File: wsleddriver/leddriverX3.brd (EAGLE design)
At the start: 100 x 38.1 mm, 55 parts, among them IC1 WS2811-SOP8, IC2 WS2811-SOP8, IC3 WS2811-SOP8

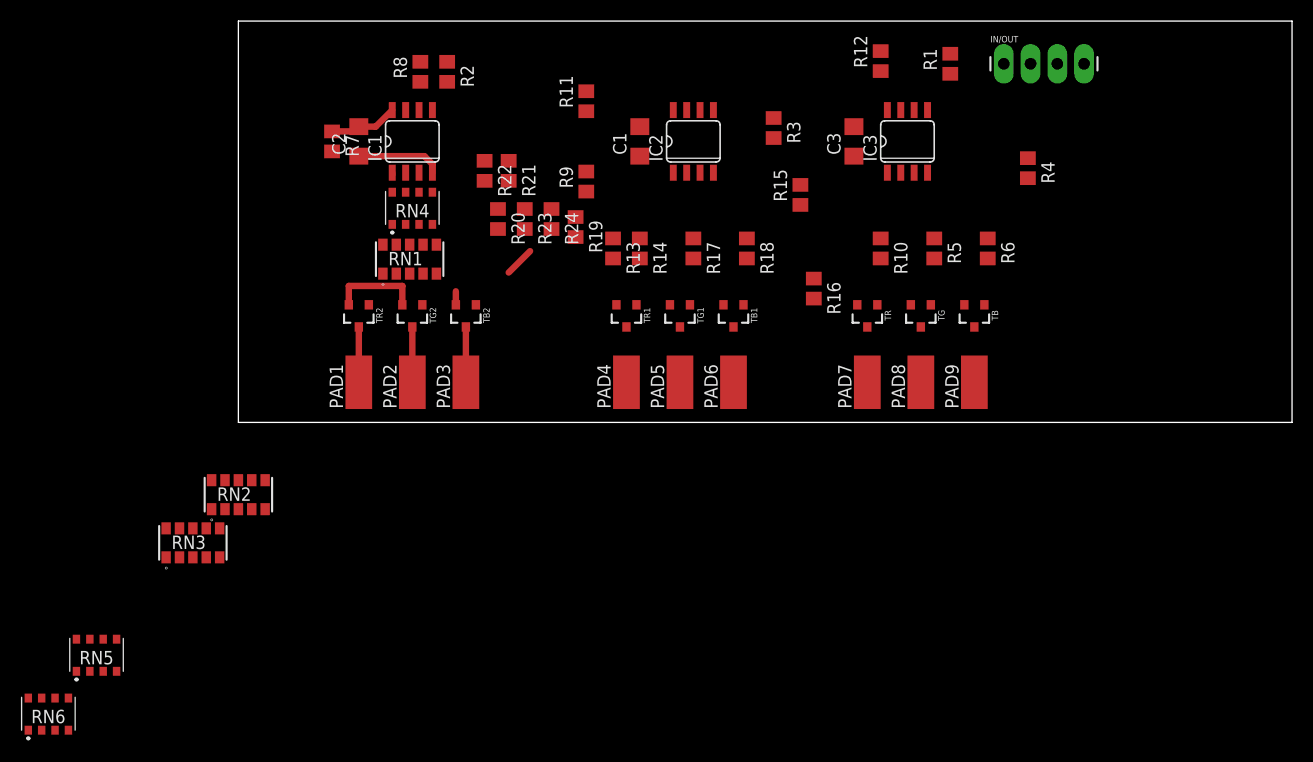
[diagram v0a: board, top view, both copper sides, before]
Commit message: h
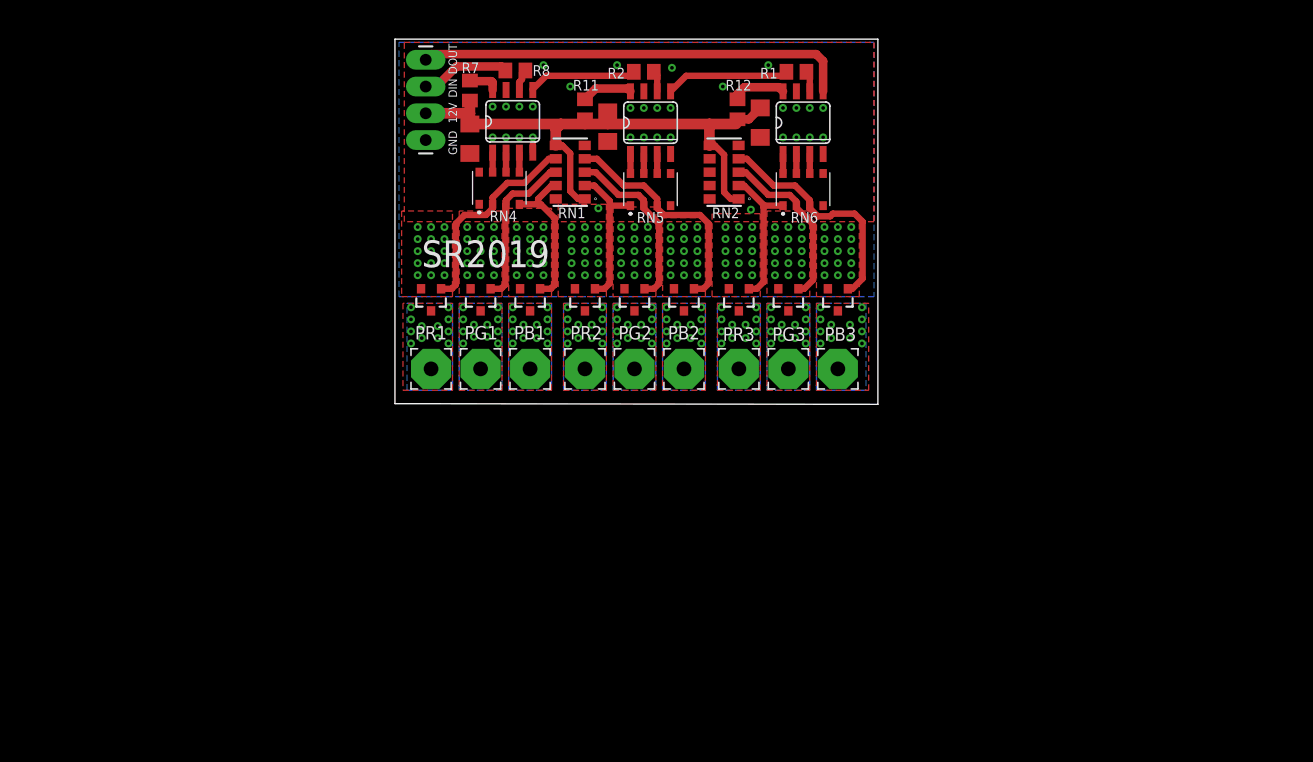
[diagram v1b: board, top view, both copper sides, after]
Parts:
- removed PAD1, PAD2, PAD3, PAD4, PAD5, PAD6, PAD7, PAD8, PAD9: (no value), wirepad:SMD2,54-5,08
- removed R10, R14, R17, R18, R20, R23, R24, R5, R6: 100, rcl:R0805
- removed R13, R15, R16, R19, R21, R22, R3, R4, R9: 10k, rcl:R0805
- removed RN3: YC358TJK-0710KL, SamacSys_Parts:YC358T
- added PB1, PB2, PB3, PG1, PG2, PG3, PR1, PR2, PR3: (no value), wirepad:3,81/1,4
- moved RN6 87.2 mm to (53.6, 22.1)
- moved RN5 68.7 mm to (39.1, 22.1)
- moved IN/OUT 55.3 mm to (17.8, 26.8), turned to 90 degrees
- moved RN2 55.3 mm to (46.1, 23.7), turned to 90 degrees
- moved R2 18.7 mm to (38.5, 33.3), turned to 180 degrees
- moved RN1 17.3 mm to (31.5, 23.7), turned to 90 degrees
- moved R1 14.6 mm to (53.0, 33.3), turned to 180 degrees
- moved R12 14.3 mm to (47.4, 29.7), turned to 270 degrees
- moved R7 13.9 mm to (22.0, 31.5)
- moved TB 13.0 mm to (56.9, 11.7)
- moved TG 12.7 mm to (52.2, 11.7)
- moved TR 12.3 mm to (47.5, 11.7)
- moved C2 10.5 mm to (22.0, 26.9)
- moved IC3 10.1 mm to (53.6, 28.4)
- moved IC1 9.71 mm to (26.0, 28.6)
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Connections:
- removed net N$10: R21.2, R23.2, TG2.1
- removed net N$12: R22.2, R24.2, TB2.1
- removed net N$15: RN1.2, RN1.7, RN4.3
- removed net N$16: RN1.3, RN1.8, RN4.2
- removed net N$17: RN1.4, RN1.9, RN4.1
- removed net N$2: R3.2, R5.2, TG.1
- removed net N$3: R4.2, R6.2, TB.1
- removed net N$4: R10.2, R9.2, TR.1
- removed net N$6: R13.2, R14.2, TR1.1
- removed net N$7: R15.2, R17.2, TG1.1
- removed net N$8: R16.2, R18.2, TB1.1
- removed net N$9: R19.2, R20.2, TR2.1
- new net TB: RN1.9, RN4.4, TB2.1
- new net TB2: RN1.4, RN5.3, TB1.1
- new net TB3: RN2.4, RN6.3, TB.1
- new net TG: RN1.8, RN4.3, TG2.1
- new net TG2: RN1.3, RN5.2, TG1.1
- new net TG3: RN2.3, RN6.2, TG.1
- new net TR: RN1.7, RN4.2, TR2.1
- new net TR2: RN1.2, RN5.1, TR1.1
- new net TR3: RN2.2, RN6.1, TR.1
- new net VDD1: IC2.8, R11.1
- new net VDD2: IC3.8, R12.1
- net +12V: now also C1.2, C2.2, C3.2, IN/OUT.2, RN1.1, RN1.6, RN2.1, RN2.6; no longer IN/OUT.4, R13.1, R15.1, R16.1, R19.1, R21.1, R22.1, R3.1, R4.1, R9.1
- net B: now also RN4.8; no longer R24.1
- net B2: now also RN5.7; no longer R18.1
- net B3: now also RN6.7; no longer R6.1
- net DOUT_OUT: now also IN/OUT.4; no longer IN/OUT.2
- net G: now also RN4.7; no longer R23.1
- net G2: now also RN5.6; no longer R17.1
- net G3: now also RN6.6; no longer R5.1
- net NEG_B: now also PB1.1; no longer PAD3.1
- net NEG_B2: now also PB2.1
- net NEG_B3: now also PB3.1
- net NEG_G: now also PG1.1; no longer PAD2.1
- net NEG_G2: now also PG2.1
- net NEG_G3: now also PG3.1
- net NEG_R: now also PR1.1; no longer PAD1.1
- net NEG_R2: now also PR2.1
- net NEG_R3: now also PR3.1
- net R: now also RN4.6; no longer R20.1
- net R2: now also RN5.5; no longer R14.1
- net R3: now also RN6.5; no longer R10.1
- net VDD: no longer C1.2, C2.2, C3.2, IC2.8, IC3.8, R11.1, R12.1
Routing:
- net +12V: track 0.00 -> 54.9 mm
- net DOUT_OUT: track 0.00 -> 41.1 mm
- net TB2: track 0.00 -> 22.1 mm
- net TB3: track 0.00 -> 22.1 mm
- net GND: track 20.9 -> 0.81 mm, vias 0 -> 167
- net TR: track 0.00 -> 20.0 mm
- net TG2: track 0.00 -> 16.8 mm
- net TG3: track 0.00 -> 16.5 mm
- net TG: track 0.00 -> 15.4 mm
- net TB: track 0.00 -> 14.5 mm
- net TR2: track 0.00 -> 14.4 mm
- net TR3: track 0.00 -> 14.0 mm
- net N$11: track 0.00 -> 11.8 mm
- net N$5: track 0.00 -> 10.4 mm
- net DIN_IN: track 0.00 -> 8.51 mm
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- added copper zone on layer 1, net GND
- added copper zone on layer 16, net GND
- added copper zone on layer 1, net NEG_B
- added copper zone on layer 16, net NEG_B
- added copper zone on layer 1, net NEG_B2
- added copper zone on layer 16, net NEG_B2
- added copper zone on layer 1, net NEG_B3
- added copper zone on layer 16, net NEG_B3
- added copper zone on layer 1, net NEG_G
- added copper zone on layer 16, net NEG_G
- added copper zone on layer 1, net NEG_G2
- added copper zone on layer 16, net NEG_G2
- added copper zone on layer 1, net NEG_G3
- added copper zone on layer 16, net NEG_G3
- added copper zone on layer 1, net NEG_R
- added copper zone on layer 16, net NEG_R
- added copper zone on layer 1, net NEG_R2
- added copper zone on layer 16, net NEG_R2
- added copper zone on layer 1, net NEG_R3
- added copper zone on layer 16, net NEG_R3
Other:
- board size 100 x 38.1 mm -> 45.8 x 34.7 mm
- board text added: "12V"
- board text added: "DIN"
- board text added: "DOUT"
- board text added: "GND"
- board text added: "SR2019"
